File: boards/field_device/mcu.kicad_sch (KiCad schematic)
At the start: 19 parts, among them J1 Conn_01x05_Pin, J2 Conn_01x02_Pin, SW1 SW_SPST, U2 STM32C011F6Px

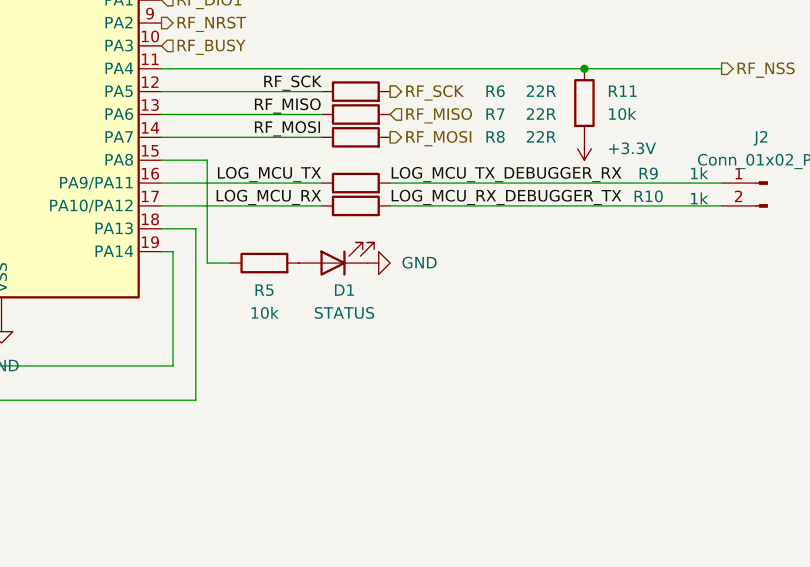
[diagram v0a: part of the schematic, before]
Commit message: i guess made schematic more readable?
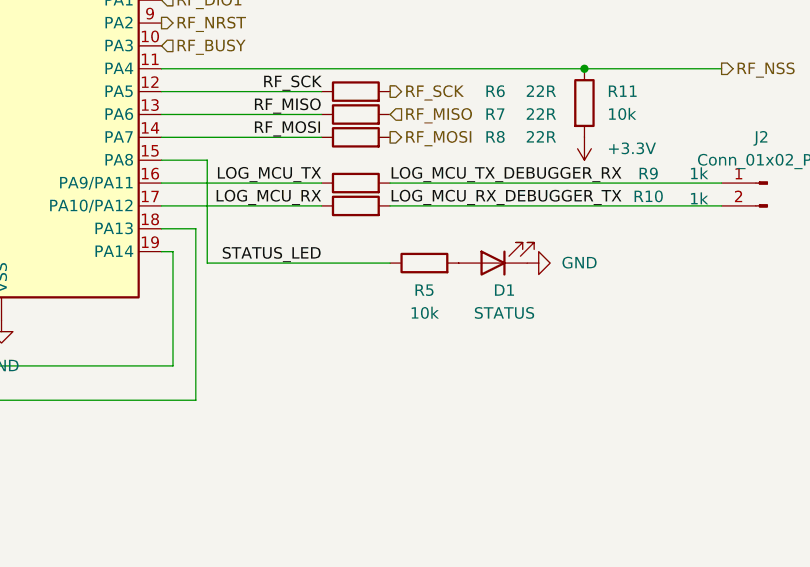
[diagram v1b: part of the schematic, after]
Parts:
- C2, C4, C5: footprint Capacitor_SMD:C_0603_1608Metric -> Capacitor_SMD:C_0603_1608Metric_Pad1.08x0.95mm_HandSolder
- C3: footprint Capacitor_SMD:C_0603_1608Metric -> Capacitor_SMD:C_0805_2012Metric_Pad1.18x1.45mm_HandSolder
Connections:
- net STATUS_LED: now reaches R5.1, U2.15 (PA8)
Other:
- moved on the sheet: D1, R5
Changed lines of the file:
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@@
 	(wire
 		(pts
-			(xy 149.86 76.2) (xy 152.4 76.2)
+			(xy 149.86 76.2) (xy 170.18 76.2)
 		)
 		(stroke
@@
 			(width 0)
 			(type default)
+		)
+	)
+	(label "STATUS_LED"
+		(at 162.56 76.2 180)
+		(effects
+			(font
+				(size 1.27 1.27)
+			)
+			(justify right bottom)
 		)
 	)
@@
 			)
 		)
-		(property "Footprint" "Capacitor_SMD:C_0603_1608Metric"
+		(property "Footprint" "Capacitor_SMD:C_0603_1608Metric_Pad1.08x0.95mm_HandSolder"
 			(at 97.4852 35.56 0)
 			(hide yes)
@@
 	(symbol
 		(lib_id "power:GND")
-		(at 167.64 76.2 90)
+		(at 185.42 76.2 90)
 		(unit 1)
 		(body_style 1)
@@
 		(fields_autoplaced yes)
 		(property "Reference" "#PWR012"
-			(at 173.99 76.2 0)
+			(at 191.77 76.2 0)
 			(hide yes)
 			(show_name no)
@@
 		)
 		(property "Value" "GND"
-			(at 171.45 76.1999 90)
+			(at 189.23 76.1999 90)
 			(show_name no)
 			(do_not_autoplace no)
@@
 		)
 		(property "Footprint" ""
-			(at 167.64 76.2 0)
-			(hide yes)
-			(show_name no)
-			(do_not_autoplace no)
-			(effects
-				(font
-					(size 1.27 1.27)
-				)
-			)
-		)
-		(property "Datasheet" ""
-			(at 167.64 76.2 0)
+			(at 185.42 76.2 0)
+			(hide yes)
+			(show_name no)
+			(do_not_autoplace no)
+			(effects
+				(font
+					(size 1.27 1.27)
+				)
+			)
+		)
+		(property "Datasheet" ""
+			(at 185.42 76.2 0)
 			(hide yes)
 			(show_name no)
@@
 		)
 		(property "Description" "Power symbol creates a global label with name \"GND\" , ground"
-			(at 167.64 76.2 0)
+			(at 185.42 76.2 0)
 			(hide yes)
 			(show_name no)
@@
 			)
 		)
-		(property "Footprint" "Capacitor_SMD:C_0603_1608Metric"
+		(property "Footprint" "Capacitor_SMD:C_0603_1608Metric_Pad1.08x0.95mm_HandSolder"
 			(at 79.7052 52.07 0)
 			(hide yes)
@@
 			)
 		)
-		(property "Footprint" "Capacitor_SMD:C_0603_1608Metric"
+		(property "Footprint" "Capacitor_SMD:C_0603_1608Metric_Pad1.08x0.95mm_HandSolder"
 			(at 111.4552 35.56 0)
 			(hide yes)
@@
 			)
 		)
-		(property "Footprint" "Capacitor_SMD:C_0603_1608Metric"
+		(property "Footprint" "Capacitor_SMD:C_0805_2012Metric_Pad1.18x1.45mm_HandSolder"
 			(at 84.7852 35.56 0)
 			(hide yes)
@@
 	(symbol
 		(lib_id "Device:LED")
-		(at 163.83 76.2 180)
+		(at 181.61 76.2 180)
 		(unit 1)
 		(body_style 1)
@@
 		(dnp no)
 		(property "Reference" "D1"
-			(at 165.1 79.248 0)
+			(at 182.88 79.248 0)
 			(show_name no)
 			(do_not_autoplace no)
@@
 		)
 		(property "Value" "STATUS"
-			(at 165.1 81.788 0)
+			(at 182.88 81.788 0)
 			(show_name no)
 			(do_not_autoplace no)
@@
 		)
 		(property "Footprint" ""
-			(at 163.83 76.2 0)
-			(hide yes)
-			(show_name no)
-			(do_not_autoplace no)
-			(effects
-				(font
-					(size 1.27 1.27)
-				)
-			)
-		)
-		(property "Datasheet" ""
-			(at 163.83 76.2 0)
+			(at 181.61 76.2 0)
+			(hide yes)
+			(show_name no)
+			(do_not_autoplace no)
+			(effects
+				(font
+					(size 1.27 1.27)
+				)
+			)
+		)
+		(property "Datasheet" ""
+			(at 181.61 76.2 0)
 			(hide yes)
 			(show_name no)
@@
 		)
 		(property "Description" "Light emitting diode"
-			(at 163.83 76.2 0)
+			(at 181.61 76.2 0)
 			(hide yes)
 			(show_name no)
@@
 		)
 		(property "Sim.Pins" "1=K 2=A"
-			(at 163.83 76.2 0)
+			(at 181.61 76.2 0)
 			(hide yes)
 			(show_name no)
@@
 	(symbol
 		(lib_id "Device:R")
-		(at 156.21 76.2 90)
+		(at 173.99 76.2 90)
 		(unit 1)
 		(body_style 1)
@@
 		(dnp no)
 		(property "Reference" "R5"
-			(at 156.21 79.248 90)
+			(at 173.99 79.248 90)
 			(show_name no)
 			(do_not_autoplace no)
@@
 		)
 		(property "Value" "10k"
-			(at 156.21 81.788 90)
+			(at 173.99 81.788 90)
 			(show_name no)
 			(do_not_autoplace no)
@@
 		)
 		(property "Footprint" ""
-			(at 156.21 77.978 90)
-			(hide yes)
-			(show_name no)
-			(do_not_autoplace no)
-			(effects
-				(font
-					(size 1.27 1.27)
-				)
-			)
-		)
-		(property "Datasheet" ""
-			(at 156.21 76.2 0)
+			(at 173.99 77.978 90)
+			(hide yes)
+			(show_name no)
+			(do_not_autoplace no)
+			(effects
+				(font
+					(size 1.27 1.27)
+				)
+			)
+		)
+		(property "Datasheet" ""
+			(at 173.99 76.2 0)
 			(hide yes)
 			(show_name no)
@@
 		)
 		(property "Description" "Resistor"
-			(at 156.21 76.2 0)
-			(hide yes)
-			(show_name no)
+			(at 173.99 76.2 0)
+			(hide yes)
+			(show_name no)
